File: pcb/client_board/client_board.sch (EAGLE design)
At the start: 18 parts, among them U1 AL5812MP-13

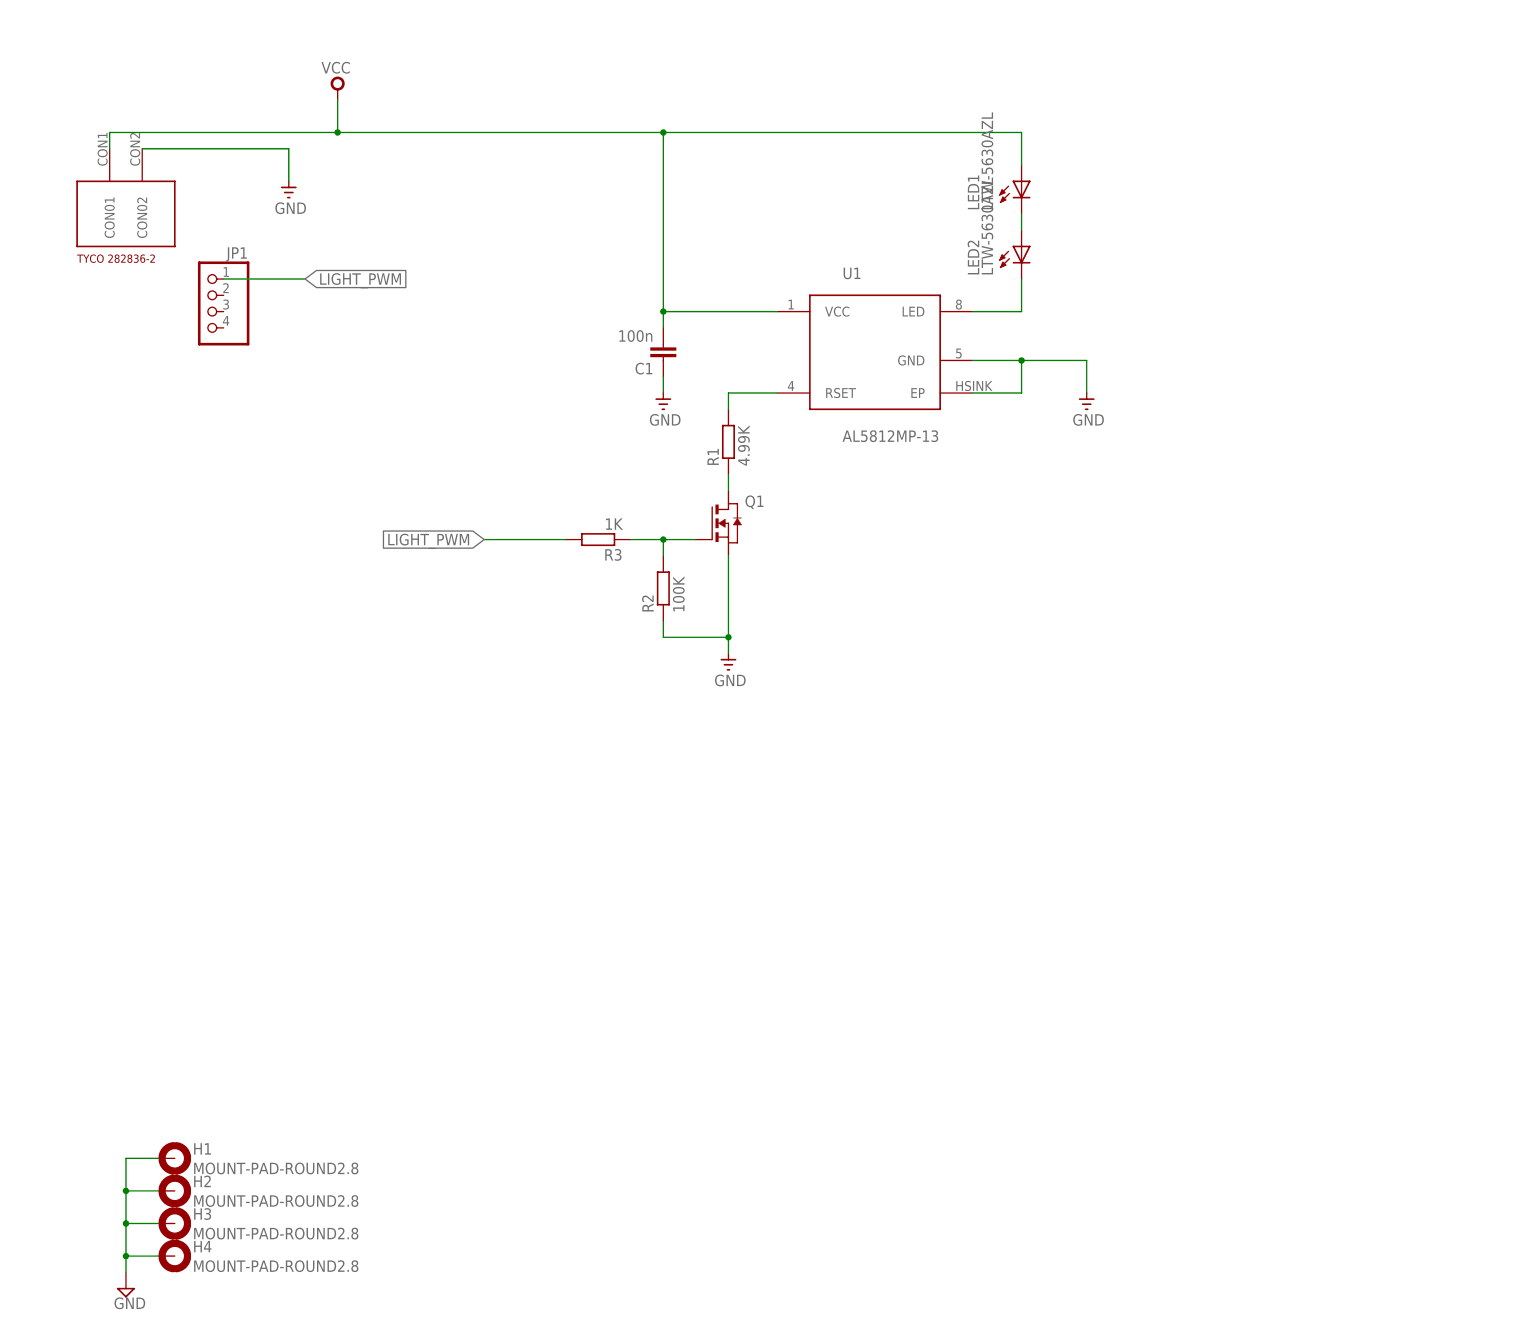
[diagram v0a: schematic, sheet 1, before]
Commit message: client board
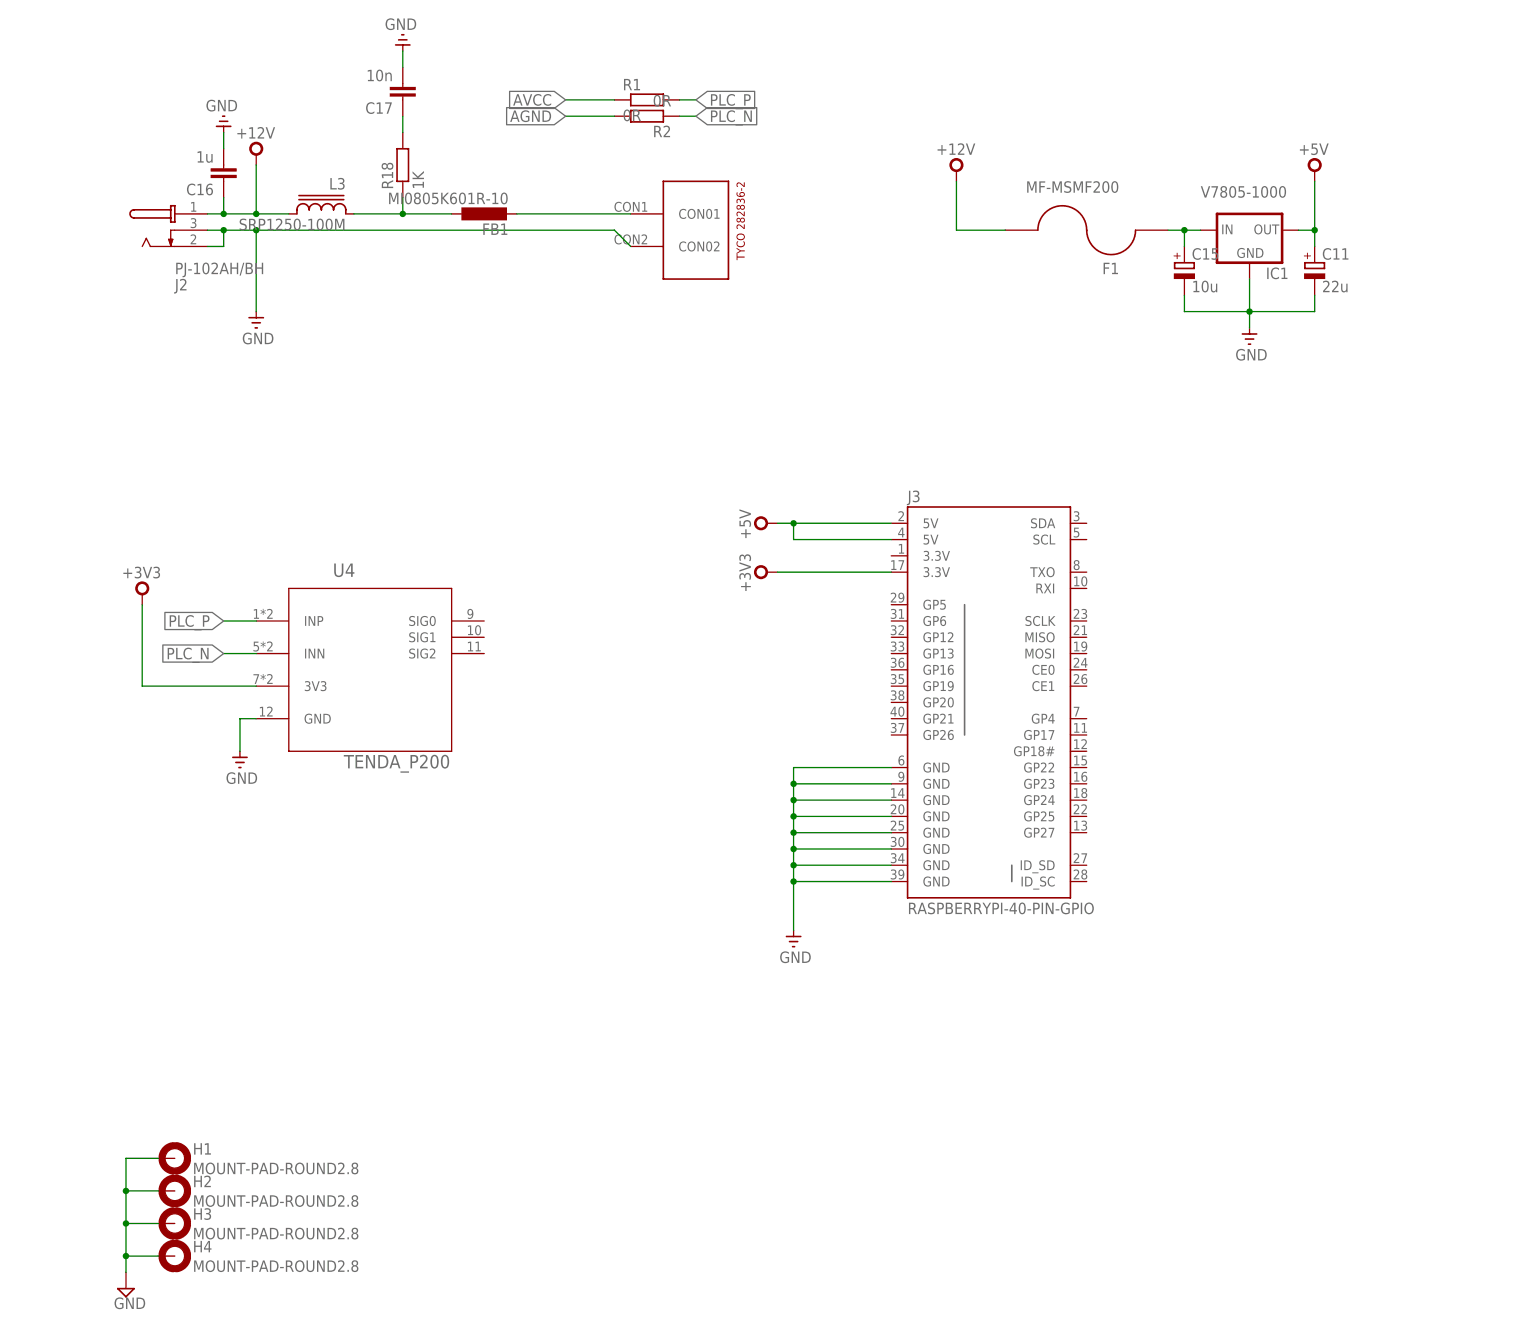
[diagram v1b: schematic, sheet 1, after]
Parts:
- removed C1: 100n, resistor:C-EUC0402
- removed C2, C3: (no value), resistor:CPOL-EU153CLV-0810
- removed ESC1, ESC2: ESC_POWER, openblw:ESC_POWER
- removed JP1: (no value), pinhead:PINHD-1X4
- removed LED1, LED2: LTW-5630AZL, openblw:LTW-5630AZL
- removed Q1: (no value), openblw:NMOS-FETSOT23
- removed R3: 1K, resistor:R-EU_R0402
- removed U1: AL5812MP-13, openblw:AL5812MP-13
- added C11: 22u, resistor:CPOL-EU153CLV-0405
- added C15: 10u, resistor:CPOL-EU153CLV-0405
- added C16: 1u, resistor:C-EUC0402
- added C17: 10n, resistor:C-EUC0402
- added F1: MF-MSMF200, openblw:MF-MSMF075/24
- added FB1: MI0805K601R-10, resistor:L-EUL5650M
- added IC1: V7805-1000, openblw:VR_1OUTXX
- added J2: PJ-102AH/BH, con-dc-power:PJ-102AH/BH
- added J3: RASPBERRYPI-40-PIN-GPIO, SparkFun-Boards:RASPBERRYPI-40-PIN-GPIO
- added L3: SRP1250-100M, openblw:SRP1250
- added R18: 1K, resistor:R-EU_R0402
- added U4: TENDA_P200, openblw:TENDA_P200
- R1: value 4.99K -> 0R; device resistor:R-EU_R0402 -> resistor:R-EU_R0603
- R2: value 100K -> 0R; device resistor:R-EU_R0402 -> resistor:R-EU_R0603
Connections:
- removed net LIGHT_PWM: JP1.1, R3.2
- removed net N$1: LED1.C, LED2.A
- removed net N$5: R1.2, U1.RSET
- removed net N$6: Q1.D, R1.1
- removed net N$7: Q1.G, R2.2, R3.1
- removed net VCC: C1.2, C2.+, C3.+, ESC1.POWER, ESC2.POWER, LED1.A, U$1.CON01, U1.VCC
- new net +12V: C16.1, F1.1, J2.T, L3.2
- new net +3V3: J3.3.3V@17, U4.3V3
- new net +5V: C11.+, IC1.OUT, J3.5V@2, J3.5V@4
- new net AGND: R2.2
- new net AVCC: R1.1
- new net AVCC_: FB1.2, U$1.CON01
- new net N$38: C17.1, R18.2
- new net N$4: C15.+, F1.2, IC1.IN
- new net PLC_N: R2.1, U4.INN
- new net PLC_P: R1.2, U4.INP
- net GND: now also C11.-, C15.-, C16.2, C17.2, IC1.GND, J2.S, J2.SS, J3.GND@14, J3.GND@20, J3.GND@25, J3.GND@30, J3.GND@34, J3.GND@39, J3.GND@6, J3.GND@9, U4.GND; no longer C1.1, C2.-, C3.-, ESC1.GND, ESC2.GND, Q1.S, R2.1, U1.EP, U1.GND
- net N$9: now also FB1.1, L3.1, R18.1; no longer LED2.C, U1.LED
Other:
- moved on the sheet: R1, R2

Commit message: before order pcbs
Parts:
- removed R1, R2: 0R, resistor:R-EU_R0603
- removed U4: TENDA_P200, openblw:TENDA_P200
- added FB2: MI0805K601R-10, resistor:L-EUL5650M
- added JP2, JP3: M20-9980346, pinhead:PINHD-2X3
- C11: value 22u -> UUD1A220MCL1GS(22u)
- C15: value 10u -> UUD1E100MCL1GS(10u)
- C16: value 1u -> EMK105BJ105KV-F(1u)
- C17: value 10n -> EMK105B7103KV-F(10n)
- F1: value MF-MSMF200 -> MF-MSMF200-2
- J2: value PJ-102AH/BH -> PJ-102AH
- J3: value RASPBERRYPI-40-PIN-GPIO -> SFH11-PBPC-D20-ST-BK
- L3: value SRP1250-100M -> SRP1245A-100M; device openblw:SRP1250 -> openblw:SRP1250A
- R18: value 1K -> ERJ-2GEJ102X(1K)
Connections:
- removed net AVCC_: FB1.2, U$1.CON01
- removed net PLC_N: R2.1, U4.INN
- removed net PLC_P: R1.2, U4.INP
- net +3V3: now also JP3.5, JP3.6; no longer U4.3V3
- net AGND: now also FB2.2, JP2.5, JP2.6, U$1.CON01; no longer R2.2
- net AVCC: now also FB1.2, JP2.1, JP2.2, U$1.CON02; no longer R1.1
- net GND: now also FB2.1, JP3.1; no longer U$1.CON02, U4.GND

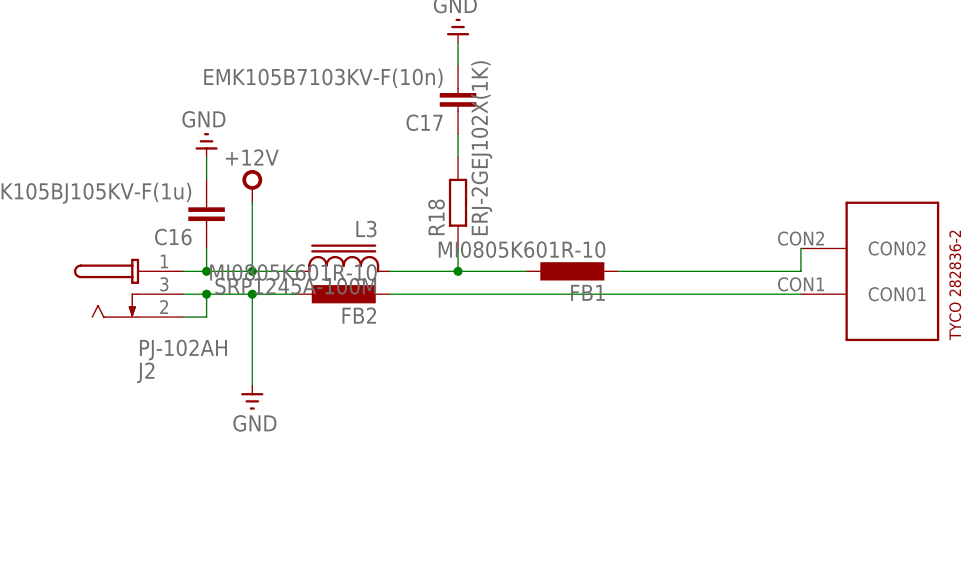
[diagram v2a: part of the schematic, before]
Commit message: parts miss
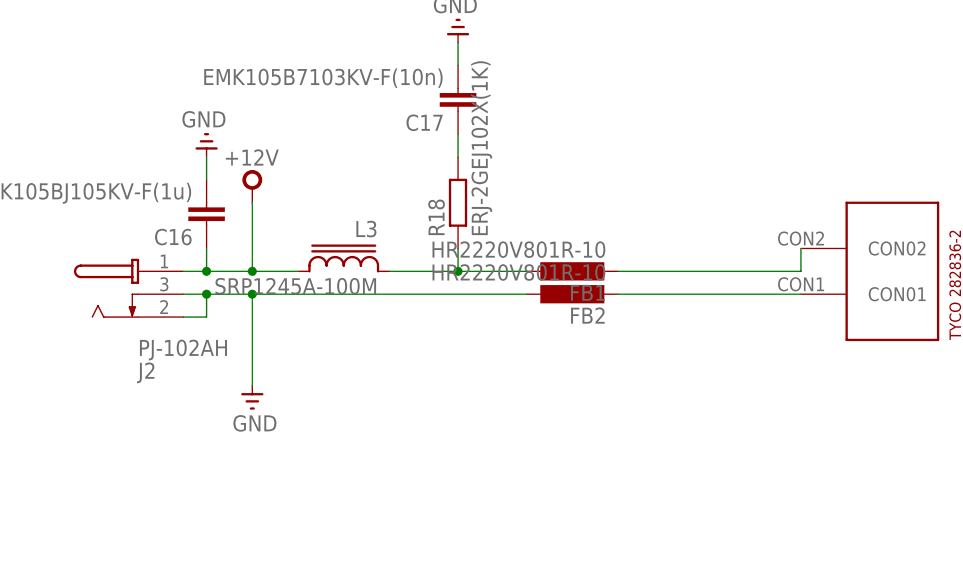
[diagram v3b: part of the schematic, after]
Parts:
- FB1, FB2: value MI0805K601R-10 -> HR2220V801R-10
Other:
- moved on the sheet: FB2
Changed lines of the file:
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@@
 <part name="V9" library="supply" deviceset="+12V" device=""/>
 <part name="C15" library="resistor" deviceset="CPOL-EU" device="153CLV-0405" value="UUD1E100MCL1GS(10u)"/>
-<part name="FB1" library="resistor" deviceset="L-EU" device="L5650M" value="MI0805K601R-10"/>
+<part name="FB1" library="resistor" deviceset="L-EU" device="L5650M" value="HR2220V801R-10"/>
 <part name="L3" library="openblw" deviceset="SRP1250A" device="" value="SRP1245A-100M"/>
 <part name="C16" library="resistor" deviceset="C-EU" device="C0402" value="EMK105BJ105KV-F(1u)"/>
@@
 <part name="V4" library="supply" deviceset="+12V" device=""/>
 <part name="J3" library="SparkFun-Boards" deviceset="RASPBERRYPI-40-PIN-GPIO" device="" value="SFH11-PBPC-D20-ST-BK"/>
-<part name="FB2" library="resistor" deviceset="L-EU" device="L5650M" value="MI0805K601R-10"/>
+<part name="FB2" library="resistor" deviceset="L-EU" device="L5650M" value="HR2220V801R-10"/>
 <part name="JP2" library="pinhead" deviceset="PINHD-2X3" device="" value="M20-9980346"/>
 <part name="JP3" library="pinhead" deviceset="PINHD-2X3" device="" value="M20-9980346"/>
@@
 <instance part="V4" gate="1" x="147.32" y="226.06"/>
 <instance part="J3" gate="G$1" x="152.4" y="144.78"/>
-<instance part="FB2" gate="G$1" x="48.26" y="215.9" rot="R90"/>
+<instance part="FB2" gate="G$1" x="73.66" y="215.9" rot="R90"/>
 <instance part="JP2" gate="A" x="38.1" y="142.24" rot="R90"/>
 <instance part="JP3" gate="A" x="71.12" y="142.24"/>
@@
 <pinref part="J2" gate="G$1" pin="S"/>
 <wire x1="30.48" y1="213.36" x2="33.02" y2="213.36" width="0.1524" layer="91"/>
-<wire x1="43.18" y1="215.9" x2="38.1" y2="215.9" width="0.1524" layer="91"/>
+<wire x1="68.58" y1="215.9" x2="38.1" y2="215.9" width="0.1524" layer="91"/>
 <junction x="33.02" y="215.9"/>
 <pinref part="GND10" gate="1" pin="GND"/>
@@
 <net name="AGND" class="2">
 <segment>
-<wire x1="99.06" y1="215.9" x2="53.34" y2="215.9" width="0.1524" layer="91"/>
+<wire x1="99.06" y1="215.9" x2="78.74" y2="215.9" width="0.1524" layer="91"/>
 <pinref part="FB2" gate="G$1" pin="2"/>
 <pinref part="U$1" gate="G$1" pin="CON01"/>
